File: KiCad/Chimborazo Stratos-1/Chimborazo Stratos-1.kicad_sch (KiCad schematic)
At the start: 7 parts, among them J1 BMP280, J2 MPU6050, J3 Conn_01x03_Pin, J4 Conn_01x03_Pin, U1 XIAO-RP2040-DIP

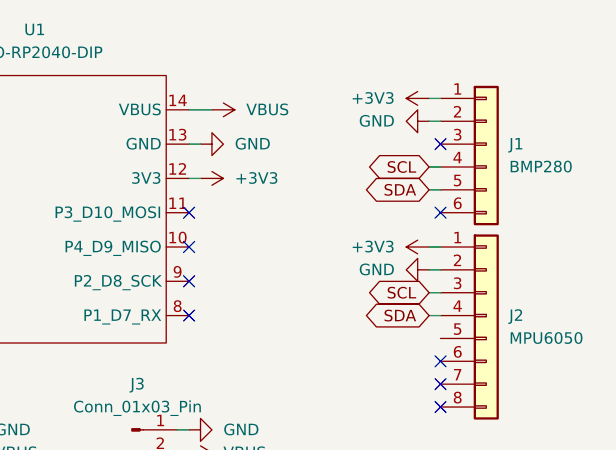
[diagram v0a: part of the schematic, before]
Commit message: Finished the pcb and the cad model REAL NO FAKE
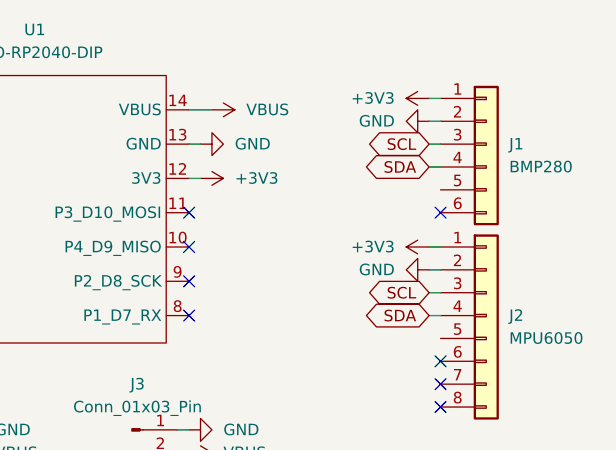
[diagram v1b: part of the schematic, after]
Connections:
- net SCL: now also J1.3 (Pin_3); no longer J1.4 (Pin_4)
- net SDA: now also J1.4 (Pin_4); no longer J1.5 (Pin_5)
- no-connect marks 11 -> 10
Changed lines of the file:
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@@
-	)
-	(no_connect
-		(at 181.61 52.07)
 	)
 	(no_connect
@@
 	(wire
 		(pts
+			(xy 180.34 52.07) (xy 181.61 52.07)
+		)
+		(stroke
+			(width 0)
+			(type default)
+		)
+	)
+	(wire
+		(pts
 			(xy 180.34 54.61) (xy 181.61 54.61)
 		)
@@
 	(wire
 		(pts
-			(xy 180.34 57.15) (xy 181.61 57.15)
-		)
-		(stroke
-			(width 0)
-			(type default)
-		)
-	)
-	(wire
-		(pts
 			(xy 95.25 59.69) (xy 100.33 59.69)
 		)
@@
 			(width 0)
 			(type default)
-		)
-	)
-	(global_label "SDA"
-		(shape bidirectional)
-		(at 180.34 57.15 180)
-		(fields_autoplaced yes)
-		(effects
-			(font
-				(size 1.27 1.27)
-			)
-			(justify right)
-		)
-		(property "Intersheetrefs" "${INTERSHEET_REFS}"
-			(at 172.6754 57.15 0)
-			(effects
-				(font
-					(size 1.27 1.27)
-				)
-				(justify right)
-				(hide yes)
-			)
 		)
 	)
@@
 		)
 	)
+	(global_label "SDA"
+		(shape bidirectional)
+		(at 180.34 54.61 180)
+		(fields_autoplaced yes)
+		(effects
+			(font
+				(size 1.27 1.27)
+			)
+			(justify right)
+		)
+		(property "Intersheetrefs" "${INTERSHEET_REFS}"
+			(at 172.6754 54.61 0)
+			(effects
+				(font
+					(size 1.27 1.27)
+				)
+				(justify right)
+				(hide yes)
+			)
+		)
+	)
+	(global_label "SCL"
+		(shape bidirectional)
+		(at 180.34 52.07 180)
+		(fields_autoplaced yes)
+		(effects
+			(font
+				(size 1.27 1.27)
+			)
+			(justify right)
+		)
+		(property "Intersheetrefs" "${INTERSHEET_REFS}"
+			(at 172.7359 52.07 0)
+			(effects
+				(font
+					(size 1.27 1.27)
+				)
+				(justify right)
+				(hide yes)
+			)
+		)
+	)
 	(global_label "PWM_2"
 		(shape output)
@@
 			(effects
 				(font
-					(size 1.27 1.27)
-				)
-				(justify right)
-				(hide yes)
-			)
-		)
-	)
-	(global_label "SCL"
-		(shape bidirectional)
-		(at 180.34 54.61 180)
-		(fields_autoplaced yes)
-		(effects
-			(font
-				(size 1.27 1.27)
-			)
-			(justify right)
-		)
-		(property "Intersheetrefs" "${INTERSHEET_REFS}"
-			(at 172.7359 54.61 0)
-			(effects
-				(font

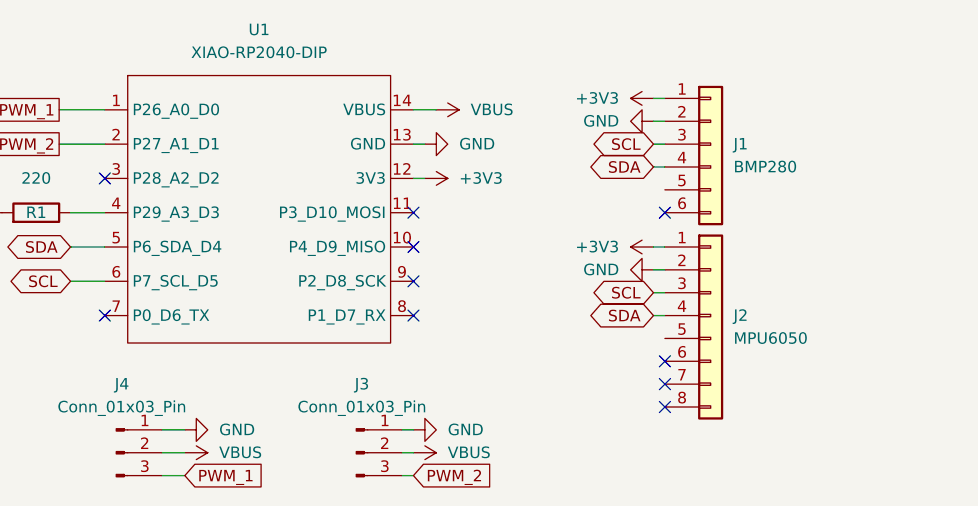
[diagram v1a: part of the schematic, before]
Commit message: Reorganized folders and Added the GERBERS files
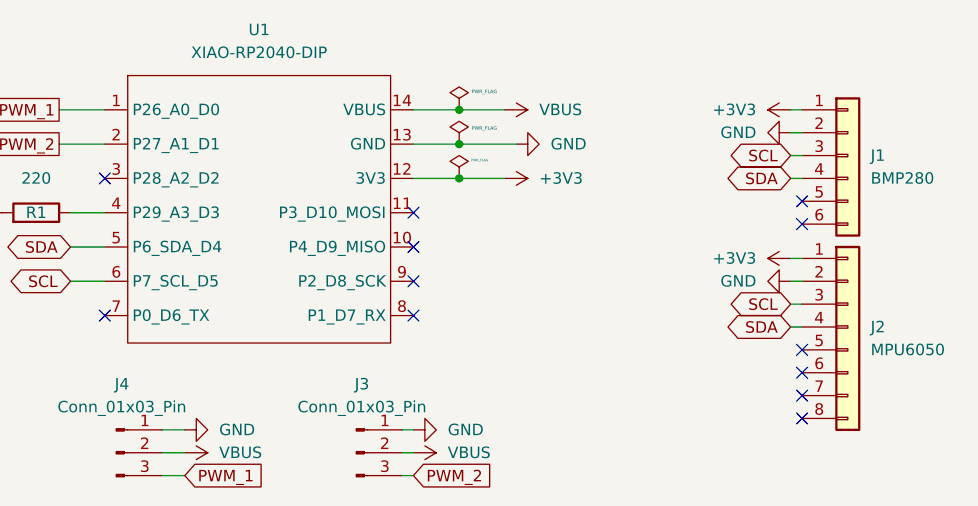
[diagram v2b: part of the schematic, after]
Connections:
- no-connect marks 10 -> 12
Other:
- moved on the sheet: J1, J2

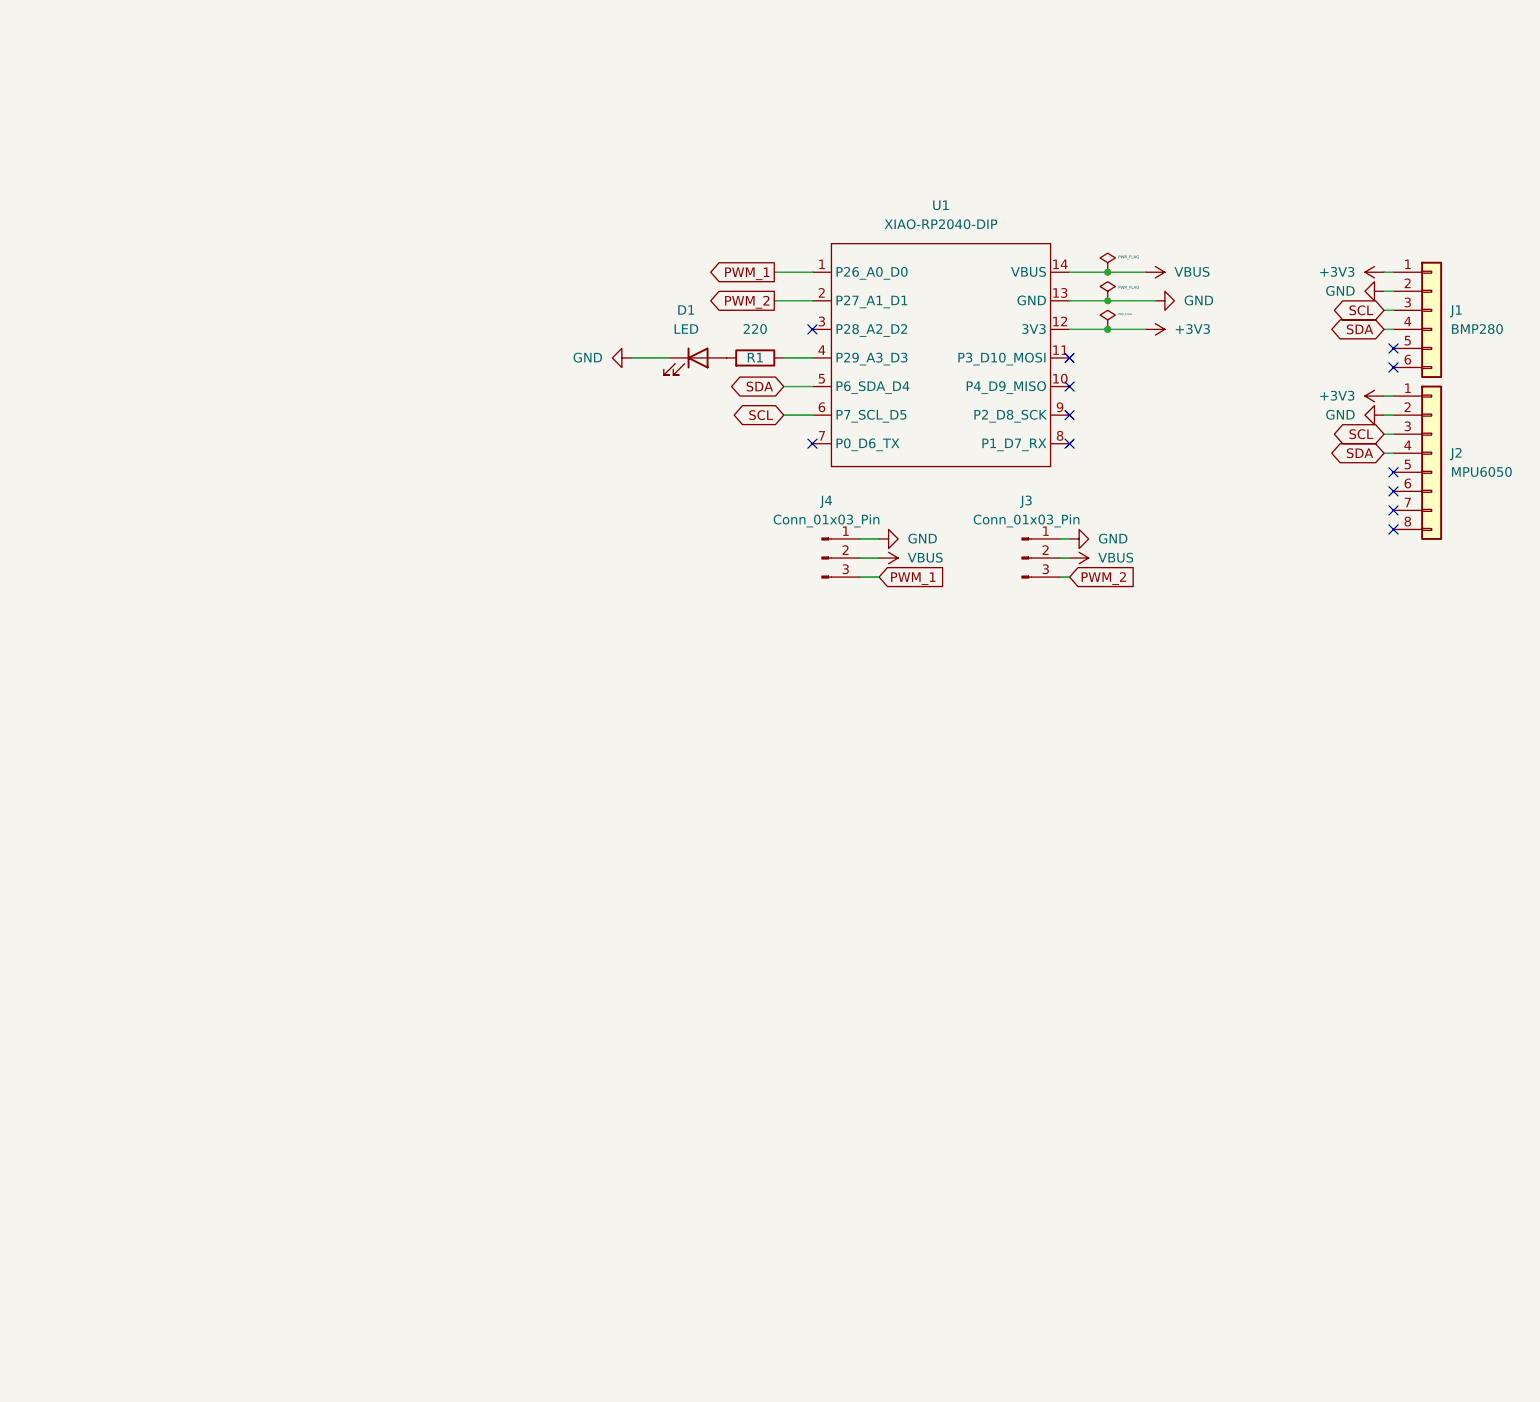
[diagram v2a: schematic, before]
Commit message: Remade schmeatic changed components and Remade PCB with new and improved layout
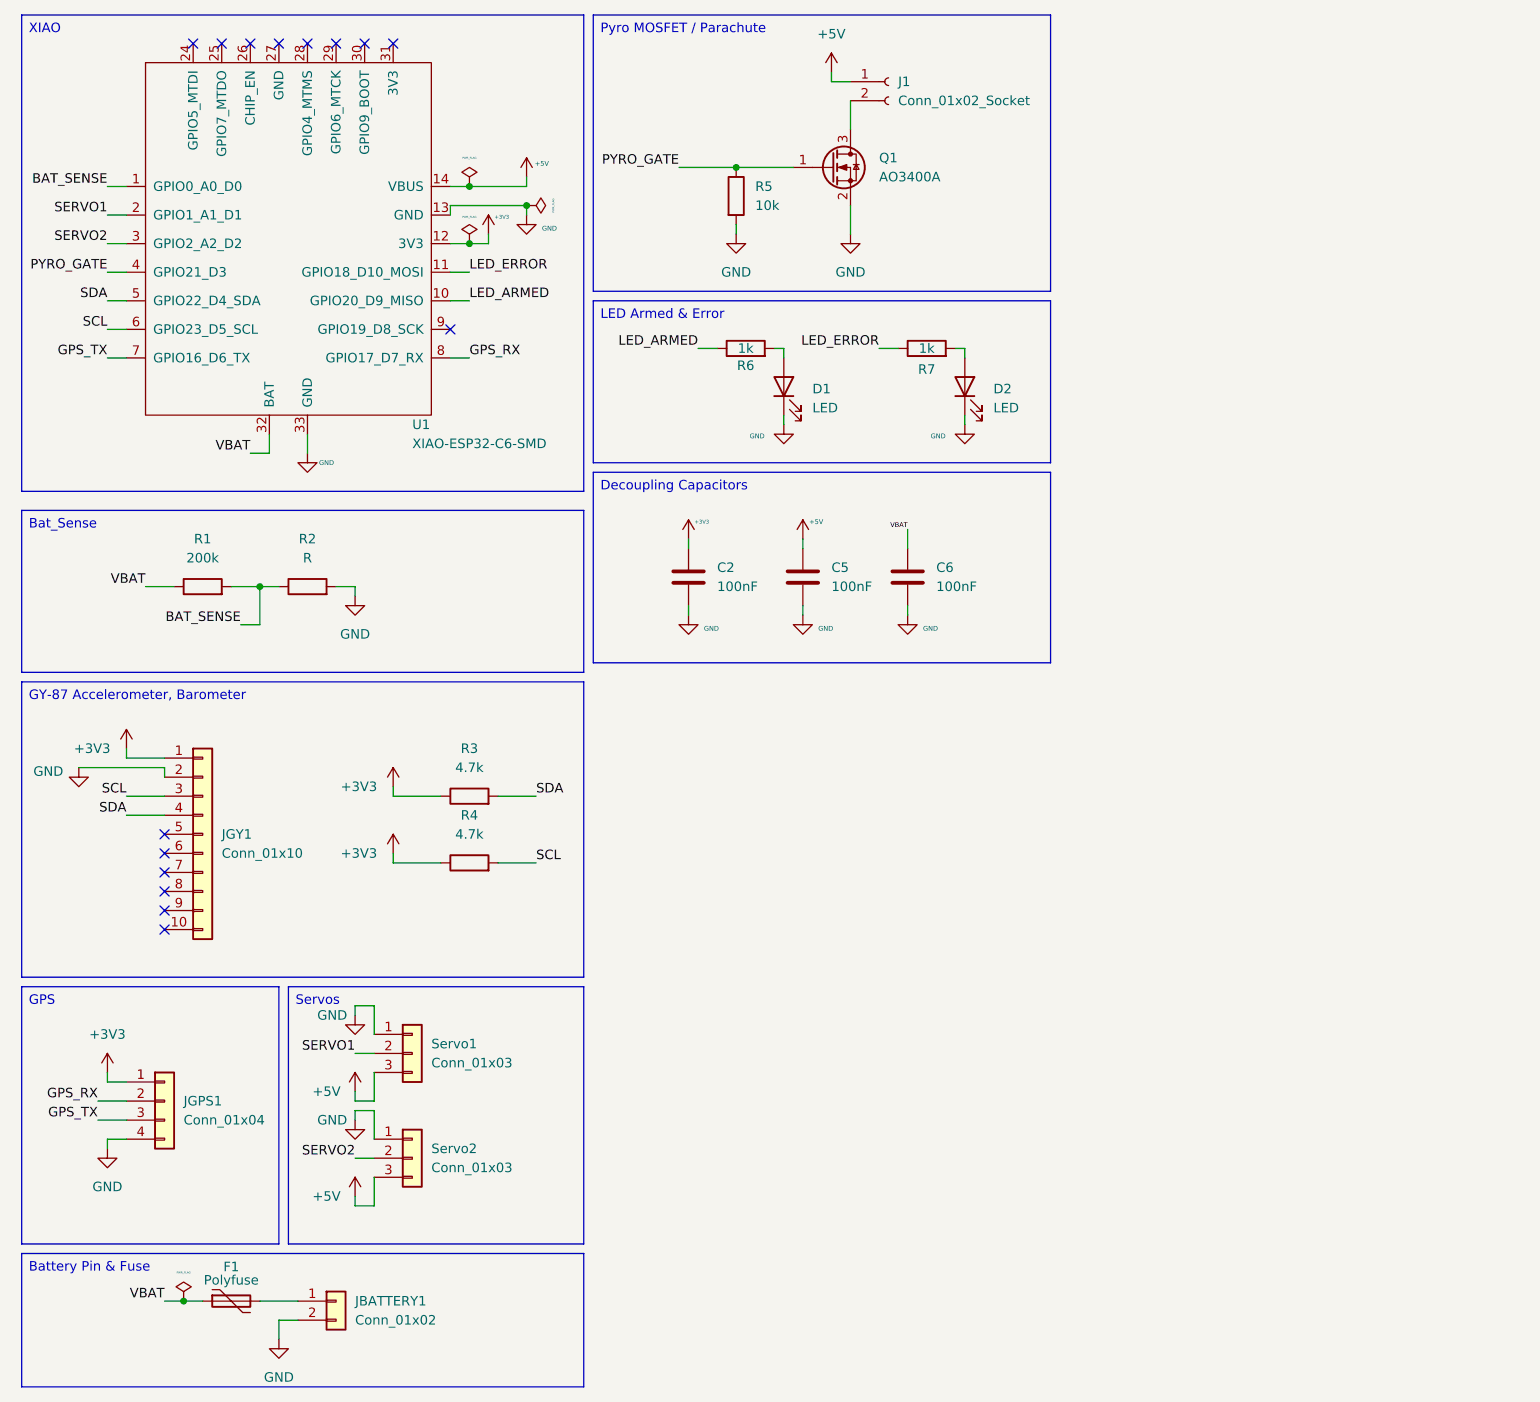
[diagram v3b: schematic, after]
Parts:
- removed J1: BMP280, Connector_PinHeader_2.54mm:PinHeader_1x06_P2.54mm_Vertical, symbol Connector_Generic:Conn_01x06
- removed J2: MPU6050, Connector_PinHeader_2.54mm:PinHeader_1x08_P2.54mm_Vertical, symbol Connector_Generic:Conn_01x08
- removed J3, J4: Conn_01x03_Pin, Connector:FanPinHeader_1x03_P2.54mm_Vertical, symbol Connector:Conn_01x03_Pin
- removed U1: XIAO-RP2040-DIP, Seeed Studio XIAO Series Library:XIAO-RP2040-DIP, symbol Seeed_Studio_XIAO_Series:XIAO-RP2040-DIP
- added C2, C5, C6: 100nF, Capacitor_SMD:C_0805_2012Metric, symbol Device:C
- added D2: LED, LED_SMD:LED_0805_2012Metric, symbol Device:LED
- added F1: Polyfuse, Fuse:Fuse_1206_3216Metric, symbol Device:Polyfuse
- added J1: Conn_01x02_Socket, Connector_PinHeader_2.54mm:PinHeader_1x02_P2.54mm_Vertical, symbol Connector:Conn_01x02_Socket
- added JBATTERY1: Conn_01x02, Connector_JST:JST_PH_B2B-PH-K_1x02_P2.00mm_Vertical, symbol Connector_Generic:Conn_01x02
- added JGPS1: Conn_01x04, Connector_PinHeader_2.54mm:PinHeader_1x04_P2.54mm_Vertical, symbol Connector_Generic:Conn_01x04
- added JGY1: Conn_01x10, Connector_PinHeader_2.54mm:PinHeader_1x10_P2.54mm_Vertical, symbol Connector_Generic:Conn_01x10
- added Q1: AO3400A, Package_TO_SOT_SMD:SOT-23, symbol Transistor_FET:AO3400A
- added R2: R, Resistor_SMD:R_0805_2012Metric, symbol Device:R
- added R3, R4: 4.7k, Resistor_SMD:R_0805_2012Metric, symbol Device:R
- added R5: 10k, Resistor_SMD:R_0805_2012Metric, symbol Device:R
- added R6, R7: 1k, Resistor_SMD:R_0805_2012Metric, symbol Device:R
- added Servo1, Servo2: Conn_01x03, Connector_PinHeader_2.54mm:PinHeader_1x03_P2.54mm_Vertical, symbol Connector_Generic:Conn_01x03
- added U1: XIAO-ESP32-C6-SMD, xiaoesp32c6:XIAO-ESP32-C6-SMD, symbol Seeed_Studio_XIAO_Series:XIAO-ESP32-C6-SMD
- D1: footprint LED_THT:LED_D5.0mm -> LED_SMD:LED_0805_2012Metric
- R1: value 220 -> 200k; footprint Resistor_THT:R_Axial_DIN0207_L6.3mm_D2.5mm_P7.62mm_Horizontal -> Resistor_SMD:R_0805_2012Metric
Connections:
- net +3V3: now also C2.1, JGPS1.1 (Pin_1), JGY1.1 (Pin_1), R3.1, R4.1, U1.12 (3V3)
- net GND: now also C2.2, C5.2, C6.2, D2.1 (K), JBATTERY1.2 (Pin_2), JGPS1.4 (Pin_4), JGY1.2 (Pin_2), Q1.2 (S), R2.2, R5.2, Servo1.1 (Pin_1), Servo2.1 (Pin_1), U1.13 (GND), U1.33 (GND)
- net SCL: now also JGY1.3 (Pin_3), R4.2, U1.6 (GPIO23_D5_SCL)
- net SDA: now also JGY1.4 (Pin_4), R3.2, U1.5 (GPIO22_D4_SDA)
- net at D1.2 (A): now also R6.2; no longer R1.2
- net VBAT: now reaches R1.1
- net VBAT: now also C6.1, F1.1, U1.32 (BAT)
- new net: D2.2 (A), R7.2
- new net: J1.2 (Pin_2), Q1.3 (D)
- new net: F1.2, JBATTERY1.1 (Pin_1)
- new net +5V: C5.1, J1.1 (Pin_1), Servo1.3 (Pin_3), Servo2.3 (Pin_3), U1.14 (VBUS)
- new net BAT_SENSE: R1.2, R2.1, U1.1 (GPIO0_A0_D0)
- new net GPS_RX: JGPS1.2 (Pin_2), U1.8 (GPIO17_D7_RX)
- new net GPS_TX: JGPS1.3 (Pin_3), U1.7 (GPIO16_D6_TX)
- new net LED_ARMED: R6.1, U1.10 (GPIO20_D9_MISO)
- new net LED_ERROR: R7.1, U1.11 (GPIO18_D10_MOSI)
- new net PYRO_GATE: Q1.1 (G), R5.1, U1.4 (GPIO21_D3)
- new net SERVO1: Servo1.2 (Pin_2), U1.2 (GPIO1_A1_D1)
- new net SERVO2: Servo2.2 (Pin_2), U1.3 (GPIO2_A2_D2)
- no-connect marks 12 -> 15
